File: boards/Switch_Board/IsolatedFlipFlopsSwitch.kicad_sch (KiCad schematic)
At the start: 12 parts, among them IC1 ISO6520FDR, J1 Screw_Terminal_01x02, U16 PTPS22811LRPWR, U3 74AUP1G79

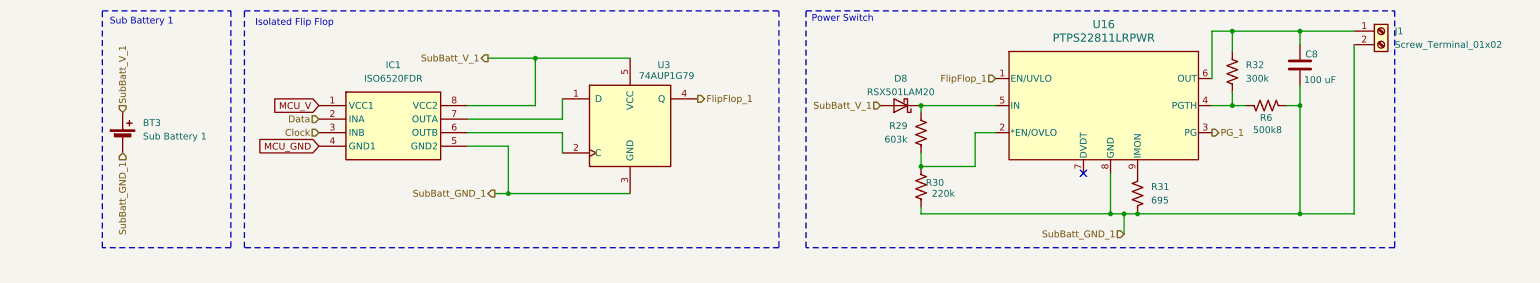
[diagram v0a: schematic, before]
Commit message: updating schematic
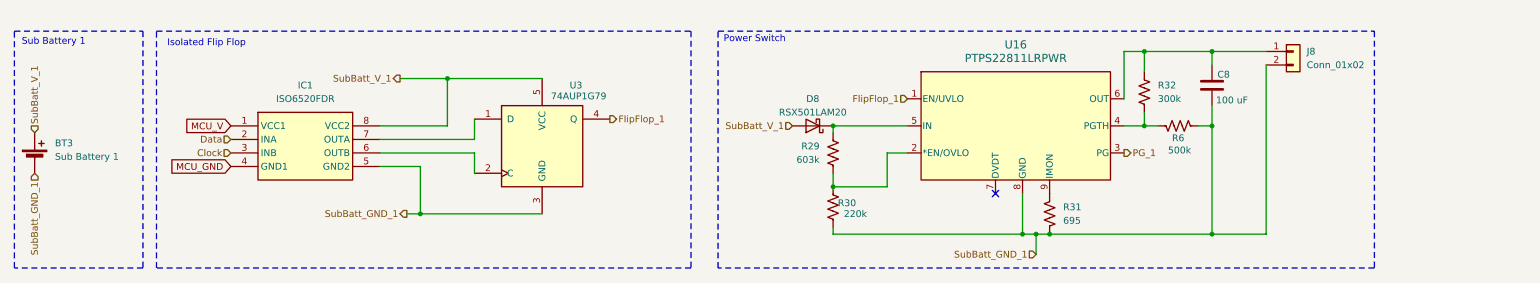
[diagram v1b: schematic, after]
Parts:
- removed J1: Screw_Terminal_01x02, Resistor_THT:R_Axial_DIN0204_L3.6mm_D1.6mm_P5.08mm_Horizontal, symbol Connector:Screw_Terminal_01x02
- added J8: Conn_01x02, symbol Connector_Generic:Conn_01x02
- renumbered 500k8 to 500k
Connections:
- net SubBatt_GND_1: now also J8.2 (Pin_2)
- net at C8.1, R32.1, U16.6 (OUT): now also J8.1 (Pin_1)
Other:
- moved on the sheet: 500k, BT3, C8, D8, IC1, R29, R30, R31, R32, U16, U3
